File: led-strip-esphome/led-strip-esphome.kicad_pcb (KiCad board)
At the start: 2 copper layers, 220 x 28 mm, 47 parts, among them Q1 FS8205A_C2830320, SW1 TS-1002S-04526C, U1 TP4056_C725790, U2 BL8072COTR33, U3 AI-WB2-12F, U4 LGS63042, U5 DW01A, U6 XDM254-1-02-W-8.5-G0

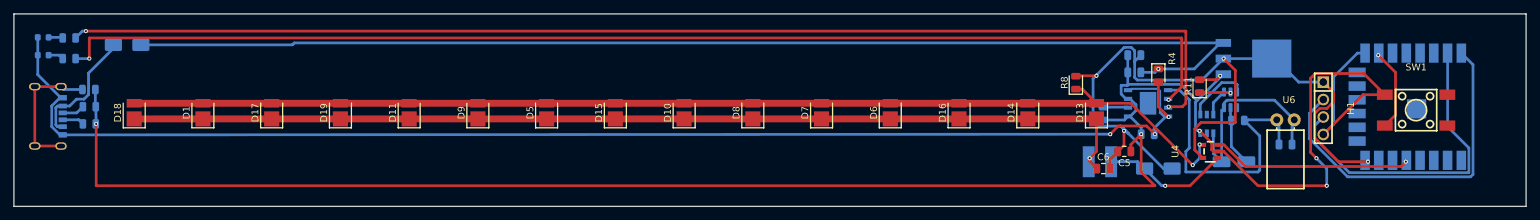
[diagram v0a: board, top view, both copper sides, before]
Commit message: update
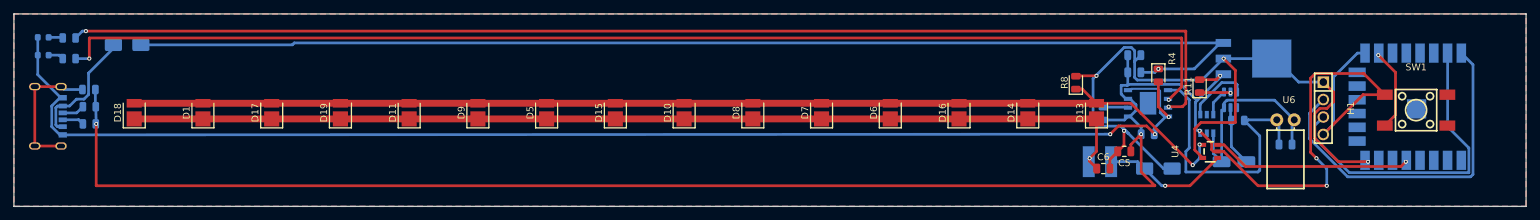
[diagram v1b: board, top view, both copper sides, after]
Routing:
- added copper zone on B.Cu, net GND
- added copper zone on F.Cu, net GND
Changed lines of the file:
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@@
 		(at 218.5 47)
 		(property "Reference" "SW1"
-			(at 0 -6.25 360)
+			(at 0 -6.25 0)
 			(layer "F.SilkS")
 			(effects
@@
 		)
 		(property "Value" "TS-1002S-04526C"
-			(at 0 6.25 360)
+			(at 0 6.25 0)
 			(layer "F.Fab")
 			(effects
@@
 		)
 		(property "Footprint" "easyeda2kicad:SW-SMD_4P-L6.0-W6.0-P4.50-LS9.0-2"
-			(at 0 0 360)
+			(at 0 0 0)
 			(layer "F.Fab")
 			(hide yes)
@@
 		)
 		(property "Datasheet" "https://lcsc.com/product-detail/Tactile-Switches_XUNPU-TS-1002S-04526C_C455109.html"
-			(at 0 0 360)
+			(at 0 0 0)
 			(layer "F.Fab")
 			(hide yes)
@@
 		)
 		(property "Description" ""
-			(at 0 0 360)
+			(at 0 0 0)
 			(layer "F.Fab")
 			(hide yes)
@@
 		)
 		(fp_text user "${REFERENCE}"
-			(at 0 0 360)
+			(at 0 0 0)
 			(layer "F.Fab")
 			(effects
@@
 		(tags "capacitor")
 		(property "Reference" "C5"
-			(at 0 -1.68 360)
+			(at 0 -1.68 0)
 			(layer "F.SilkS")
 			(effects
@@
 		)
 		(property "Value" "4.7uF"
-			(at 0 1.68 360)
+			(at 0 1.68 0)
 			(layer "F.Fab")
 			(effects
@@
 		)
 		(fp_text user "${REFERENCE}"
-			(at 0 0 360)
+			(at 0 0 0)
 			(layer "F.Fab")
 			(effects
@@
 		(tags "capacitor")
 		(property "Reference" "C2"
-			(at 0 1.68 360)
+			(at 0 1.68 0)
 			(layer "B.SilkS")
 			(effects
@@
 		)
 		(property "Value" "10uF"
-			(at 0 -1.68 360)
+			(at 0 -1.68 0)
 			(layer "B.Fab")
 			(effects
@@
 		)
 		(fp_text user "${REFERENCE}"
-			(at 0 0 360)
+			(at 0 0 0)
 			(layer "B.Fab")
 			(effects
@@
 		(tags "LED")
 		(property "Reference" "R7"
-			(at 2.52869 0 360)
+			(at 2.52869 0 0)
 			(layer "B.SilkS")
 			(effects
@@
 		)
 		(property "Value" "5.11k"
-			(at 0 -1.65 360)
+			(at 0 -1.65 0)
 			(layer "B.Fab")
 			(effects
@@
 		)
 		(fp_text user "${REFERENCE}"
-			(at 0 0 360)
+			(at 0 0 0)
 			(layer "B.Fab")
 			(effects
@@
 		(tags "capacitor")
 		(property "Reference" "C3"
-			(at 3 0 360)
+			(at 3 0 0)
 			(layer "B.SilkS")
 			(effects
@@
 		)
 		(property "Value" "1uF"
-			(at 0 -1.68 360)
+			(at 0 -1.68 0)
 			(layer "B.Fab")
 			(effects
@@
 		)
 		(fp_text user "${REFERENCE}"
-			(at 0 0 360)
+			(at 0 0 0)
 			(layer "B.Fab")
 			(effects
@@
 		(tags "LED")
 		(property "Reference" "R2"
-			(at -0.03381 -2 360)
+			(at -0.03381 -2 0)
 			(layer "B.SilkS")
 			(effects
@@
 		)
 		(property "Value" "210"
-			(at 0 -1.65 360)
+			(at 0 -1.65 0)
 			(layer "B.Fab")
 			(effects
@@
 		)
 		(fp_text user "${REFERENCE}"
-			(at 0 0 360)
+			(at 0 0 0)
 			(layer "B.Fab")
 			(effects
@@
 		(tags "LED")
 		(property "Reference" "R5"
-			(at 2.59119 0 360)
+			(at 2.59119 0 0)
 			(layer "B.SilkS")
 			(effects
@@
 		)
 		(property "Value" "1M"
-			(at 0 -1.65 360)
+			(at 0 -1.65 0)
 			(layer "B.Fab")
 			(effects
@@
 		)
 		(fp_text user "${REFERENCE}"
-			(at 0 0 360)
+			(at 0 0 0)
 			(layer "B.Fab")
 			(effects
@@
 		(tags "capacitor")
 		(property "Reference" "C1"
-			(at 4.05 0 360)
+			(at 4.05 0 0)
 			(layer "B.SilkS")
 			(effects
@@
 		)
 		(property "Value" "10uF"
-			(at 0 -1.68 360)
+			(at 0 -1.68 0)
 			(layer "B.Fab")
 			(effects
@@
 		)
 		(fp_text user "${REFERENCE}"
-			(at 0 0 360)
+			(at 0 0 0)
 			(layer "B.Fab")
 			(effects
@@
 		(tags "smd inductor dlg-0403")
 		(property "Reference" "L1"
-			(at 0 3.2 360)
+			(at 0 3.2 0)
 			(layer "B.SilkS")
 			(effects
@@
 		)
 		(property "Value" "10uH"
-			(at 0 -3.2 360)
+			(at 0 -3.2 0)
 			(layer "B.Fab")
 			(effects
@@
 		)
 		(fp_text user "${REFERENCE}"
-			(at 0 0 360)
+			(at 0 0 0)
 			(layer "B.Fab")
 			(effects
@@
 		(tags "LED")
 		(property "Reference" "D3"
-			(at 0 1.43 360)
+			(at 0 1.43 0)
 			(layer "B.SilkS")
 			(effects
@@
 		)
 		(property "Value" "LED"
-			(at 0 -1.43 360)
+			(at 0 -1.43 0)
 			(layer "B.Fab")
 			(effects
@@
 		)
 		(fp_text user "${REFERENCE}"
-			(at 0 0 360)
+			(at 0 0 0)
 			(layer "B.Fab")
 			(effects
@@
 		(tags "LED")
 		(property "Reference" "R3"
-			(at 0 1.65 360)
+			(at 0 1.65 0)
 			(layer "B.SilkS")
 			(effects
@@
 		)
 		(property "Value" "210"
-			(at 0 -1.65 360)
+			(at 0 -1.65 0)
 			(layer "B.Fab")
 			(effects
@@
 		)
 		(fp_text user "${REFERENCE}"
-			(at 0 0 360)
+			(at 0 0 0)
 			(layer "B.Fab")
 			(effects
@@
 		(tags "LED")
 		(property "Reference" "D2"
-			(at 0 -1.5 360)
+			(at 0 -1.5 0)
 			(layer "B.SilkS")
 			(effects
@@
 		)
 		(property "Value" "LED"
-			(at 0 -1.43 360)
+			(at 0 -1.43 0)
 			(layer "B.Fab")
 			(effects
@@
 		)
 		(fp_text user "${REFERENCE}"
-			(at 0 0 360)
+			(at 0 0 0)
 			(layer "B.Fab")
 			(effects
@@
 		(tags "LED")
 		(property "Reference" "R6"
-			(at 2.52869 0 360)
+			(at 2.52869 0 0)
 			(layer "B.SilkS")
 			(effects
@@
 		)
 		(property "Value" "5.11k"
-			(at 0 -1.65 360)
+			(at 0 -1.65 0)
 			(layer "B.Fab")
 			(effects
@@
 		)
 		(fp_text user "${REFERENCE}"
-			(at 0 0 360)
+			(at 0 0 0)
 			(layer "B.Fab")
 			(effects
@@
 		(tags "capacitor")
 		(property "Reference" "C4"
-			(at -3 0 360)
+			(at -3 0 0)
 			(layer "B.SilkS")
 			(effects
@@
 		)
 		(property "Value" "1uF"
-			(at 0 -1.68 360)
+			(at 0 -1.68 0)
 			(layer "B.Fab")
 			(effects
@@
 		)
 		(fp_text user "${REFERENCE}"
-			(at 0 0 360)
+			(at 0 0 0)
 			(layer "B.Fab")
 			(effects
@@
 		(tags "Diode SMA (DO-214AC)")
 		(property "Reference" "D4"
-			(at 0 2.5 360)
+			(at 0 2.5 0)
 			(layer "B.SilkS")
 			(effects
@@
 		)
 		(property "Value" "D"
-			(at 0 -2.6 360)
+			(at 0 -2.6 0)
 			(layer "B.Fab")
 			(effects
@@
 		)
 		(fp_text user "${REFERENCE}"
-			(at 0 2.5 360)
+			(at 0 2.5 0)
 			(layer "B.Fab")
 			(effects
@@
 		(net 49)
 	)
+	(zone
+		(net 5)
+		(net_name "GND")
+		(layers "F&B.Cu")
+		(hatch edge 0.5)
+		(connect_pads
+			(clearance 0.5)
+		)
+		(min_thickness 0.25)
+		(filled_areas_thickness no)
+		(fill yes
+			(thermal_gap 0.5)
+			(thermal_bridge_width 0.5)
+		)
+		(polygon
+			(pts
+				(xy 14.5 33) (xy 14.5 61) (xy 234.5 61) (xy 234.5 33)
+			)
+		)
+	)
 )
